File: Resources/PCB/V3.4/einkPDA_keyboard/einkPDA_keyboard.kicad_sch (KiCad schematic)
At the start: 135 parts, among them J1 USB_C_Receptacle_USB2.0_16P, J2 Conn_01x12_Pin, J3 Conn_01x26_Pin, J4 Micro_SD_Card, J5 Conn_01x12_Pin, Q1 MMBT3904, SW36 YTS-C017-2B, SW4 SW_DIP_x02, SW41 YTS-C017-2B, U1 ESP32-S3-WROOM-1-N16R2, U10 TS3USB30ERSWR, U2 USBLC6-2SC6, U3 TPS63001, U4 PCF8563T, U5 TCA8418RTWR, U6 C2764211, U7 TPS61040DBV, U8 TPS22917DBV, U9 MP2722GRH-0000-Z, Y1 Crystal_32.768kHz

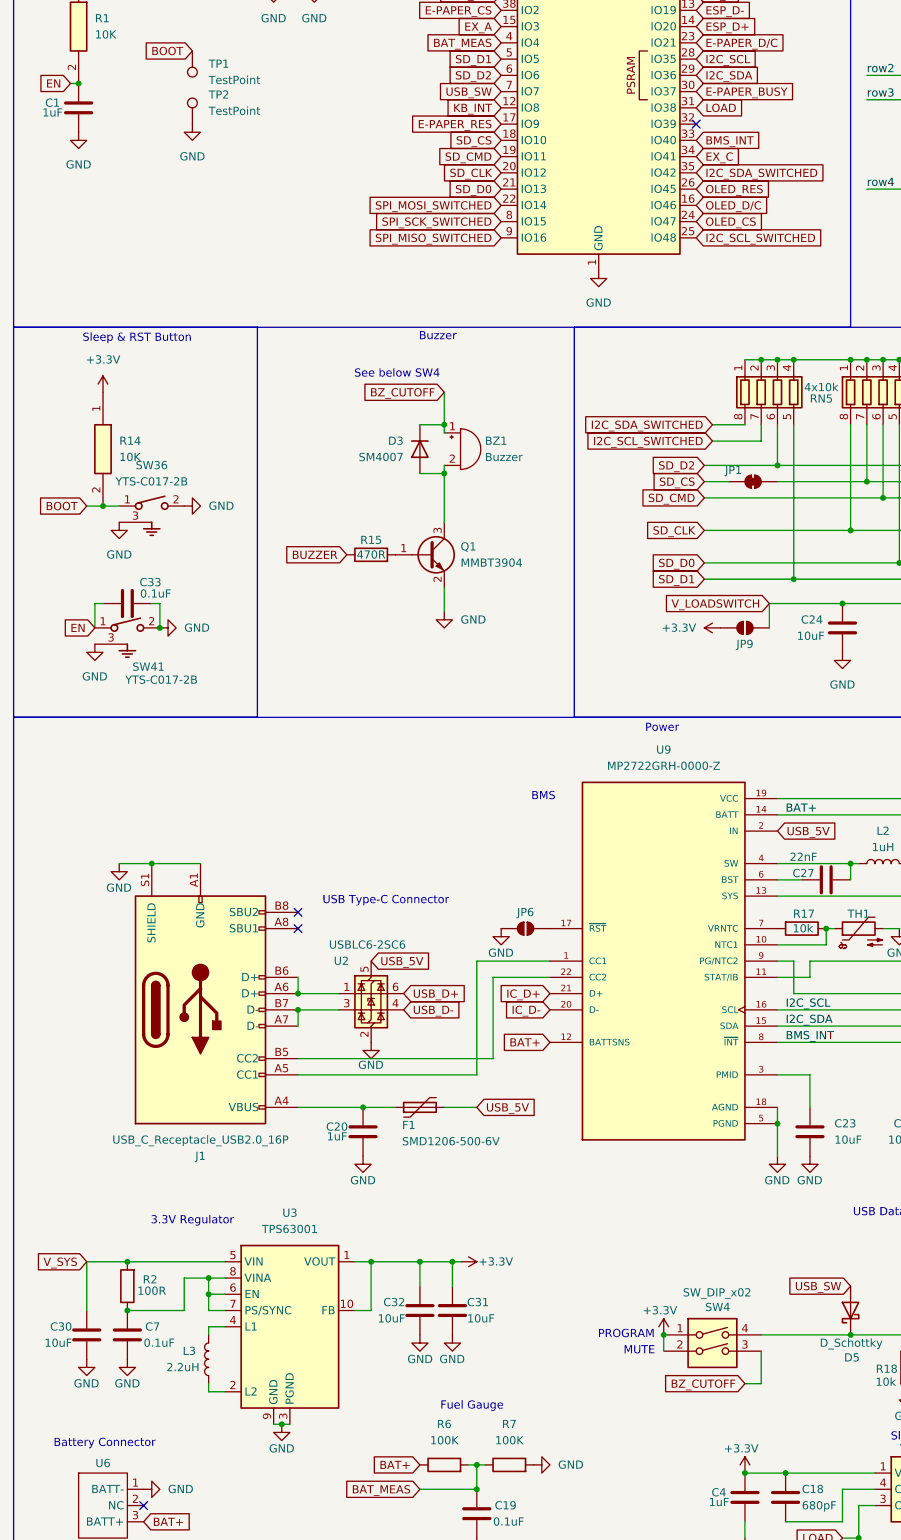
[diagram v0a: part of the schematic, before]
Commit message: Keyboard PCB power system update
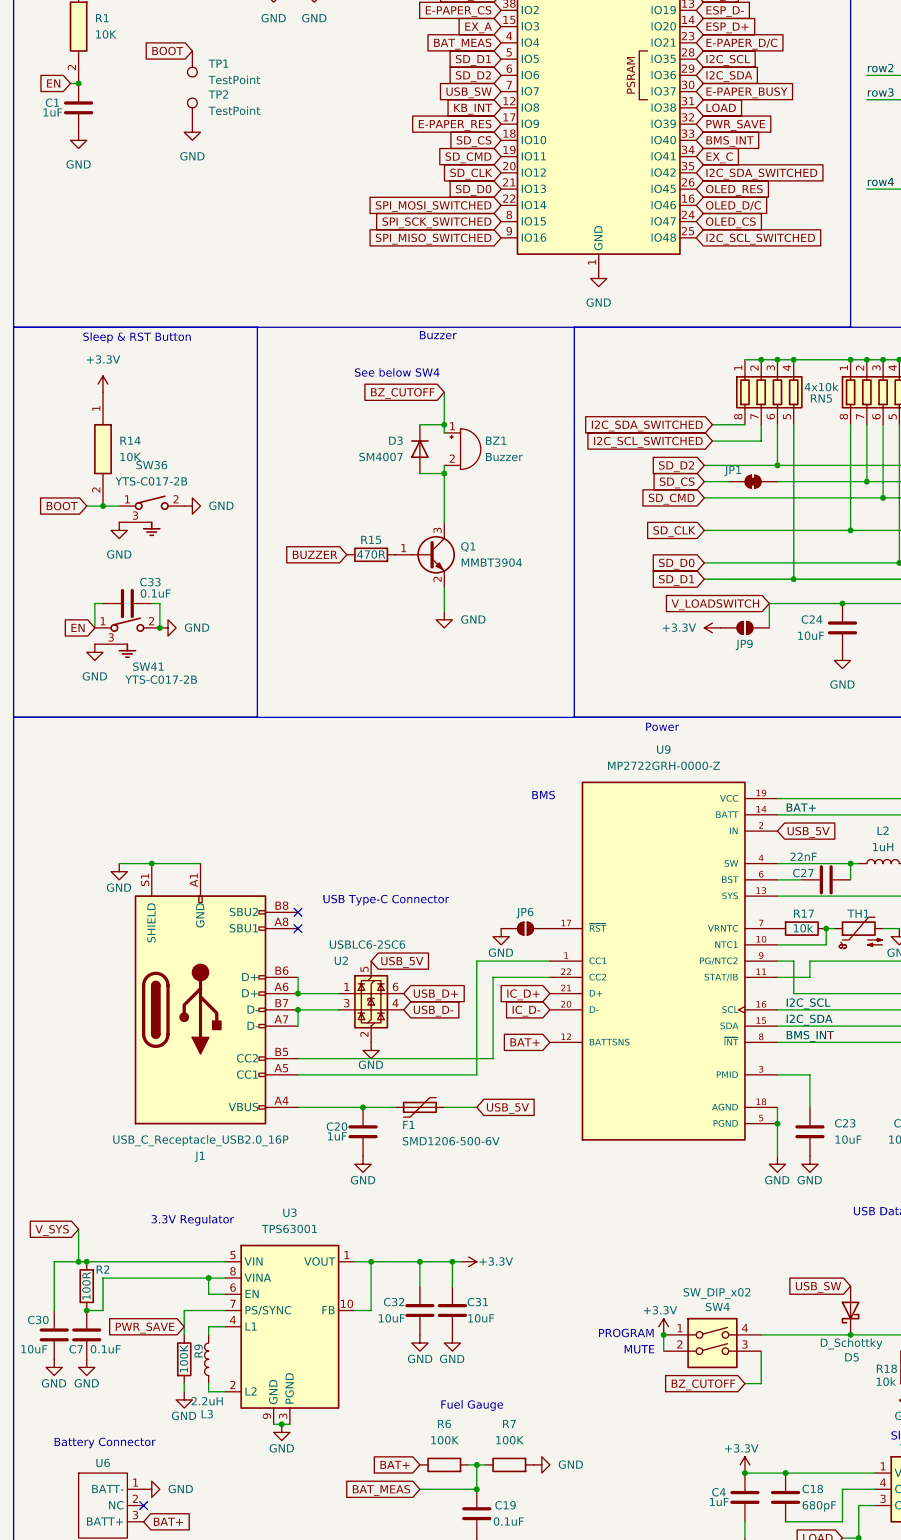
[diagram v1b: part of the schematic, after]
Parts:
- added R9: 100K, Resistor_SMD:R_0603_1608Metric, symbol Device:R
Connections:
- net GND: now also R9.2
- net at C7.1, R2.1, U3.6 (EN)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: no longer U3.7 (PS/SYNC)
- net PWR_SAVE: now reaches U1.32 (IO39)
- net PWR_SAVE: now also U3.7 (PS/SYNC), R9.1
- no-connect marks 10 -> 9
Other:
- moved on the sheet: C30, C7, R2
